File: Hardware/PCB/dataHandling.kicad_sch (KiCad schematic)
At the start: 13 parts, among them J1 USB_B, U10 74HC595, U11 74HC595, U12 74HC595, U13 MCP2221AxP, U9 74HC165

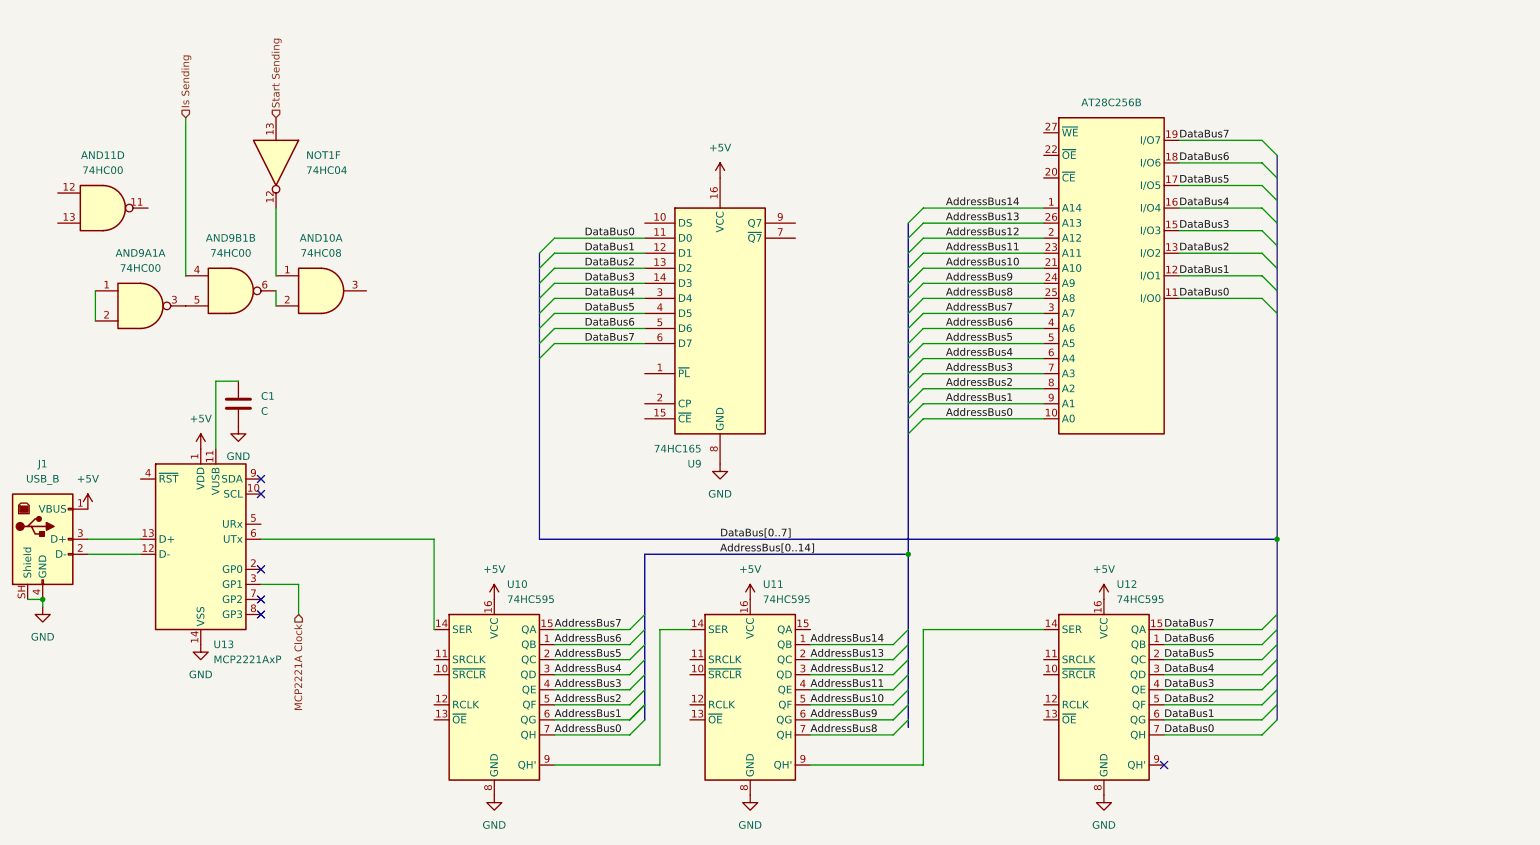
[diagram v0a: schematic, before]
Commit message: Finished schematic
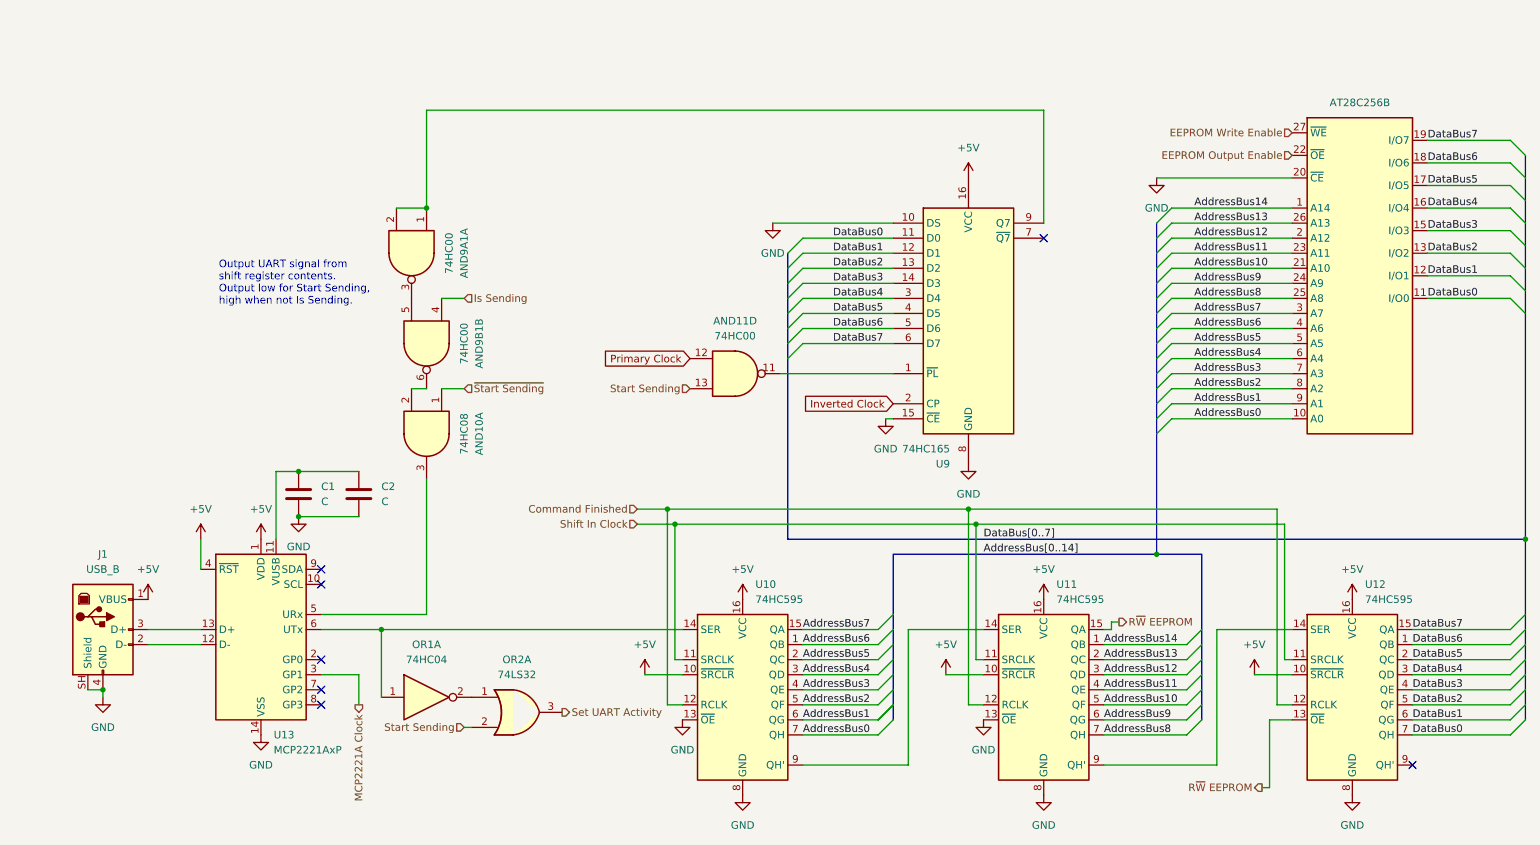
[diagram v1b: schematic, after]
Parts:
- removed NOT1: 74HC04, symbol 74xx:74HC04
- added C2: C, symbol Device:C
- added OR1: 74HC04, symbol 74xx:74HC04
- added OR2: 74LS32, symbol 74xx:74LS32
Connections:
- net +5V: now also U10.10 (~{SRCLR}), U11.10 (~{SRCLR}), U12.10 (~{SRCLR}), U13.4 (~{RST})
- net GND: now also AT28C256.20 (~{CE}), U10.13 (~{OE}), U11.13 (~{OE}), U9.10 (DS), U9.15 (~{CE}), C2.2
- net Start Sending: now also AND11.13, OR2.2
- net at C1.1, U13.11 (VUSB): now also C2.1
- net ~{Start Sending}: now reaches AND10.1
- net at AND10.3: now also U13.5 (URx)
- net at U9.1 (~{PL}): now also AND11.11
- net Inverted Clock: now reaches U9.2 (CP)
- net at U9.9 (Q7): now also AND9A1.1, AND9A1.2
- net Shift In Clock: now reaches U12.11 (SRCLK)
- net Shift In Clock: now also U10.11 (SRCLK), U11.11 (SRCLK)
- net Command Finished: now reaches U12.12 (RCLK)
- net Command Finished: now also U10.12 (RCLK), U11.12 (RCLK)
- net R~{W} EEPROM: now reaches U12.13 (~{OE})
- net R~{W} EEPROM: now also U11.15 (QA)
- net Primary Clock: now reaches AND11.12
- net at U10.14 (SER), U13.6 (UTx): now also OR1.1
- net EEPROM Output Enable: now reaches AT28C256.22 (~{OE})
- net EEPROM Write Enable: now reaches AT28C256.27 (~{WE})
- new net: OR1.2, OR2.1
- new net Set UART Activity: OR2.3
- no-connect marks 6 -> 7
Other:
- note added: "Output UART signal from shift register contents. Output low for Start Sending, high when not Is Sending."
- moved on the sheet: AND10A, AND11D, AND9A1A, AND9B1B, AT28C256B, C1, J1, U10, U11, U12, U13, U9
